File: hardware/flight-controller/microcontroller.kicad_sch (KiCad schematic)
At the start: 49 parts, among them J10 Conn_01x05, J8 IDC-6, J9 IDC-10, SW2 SW_Push, U4 STM32U535RET6, U5 ESP-12E, Y1 8 MHz

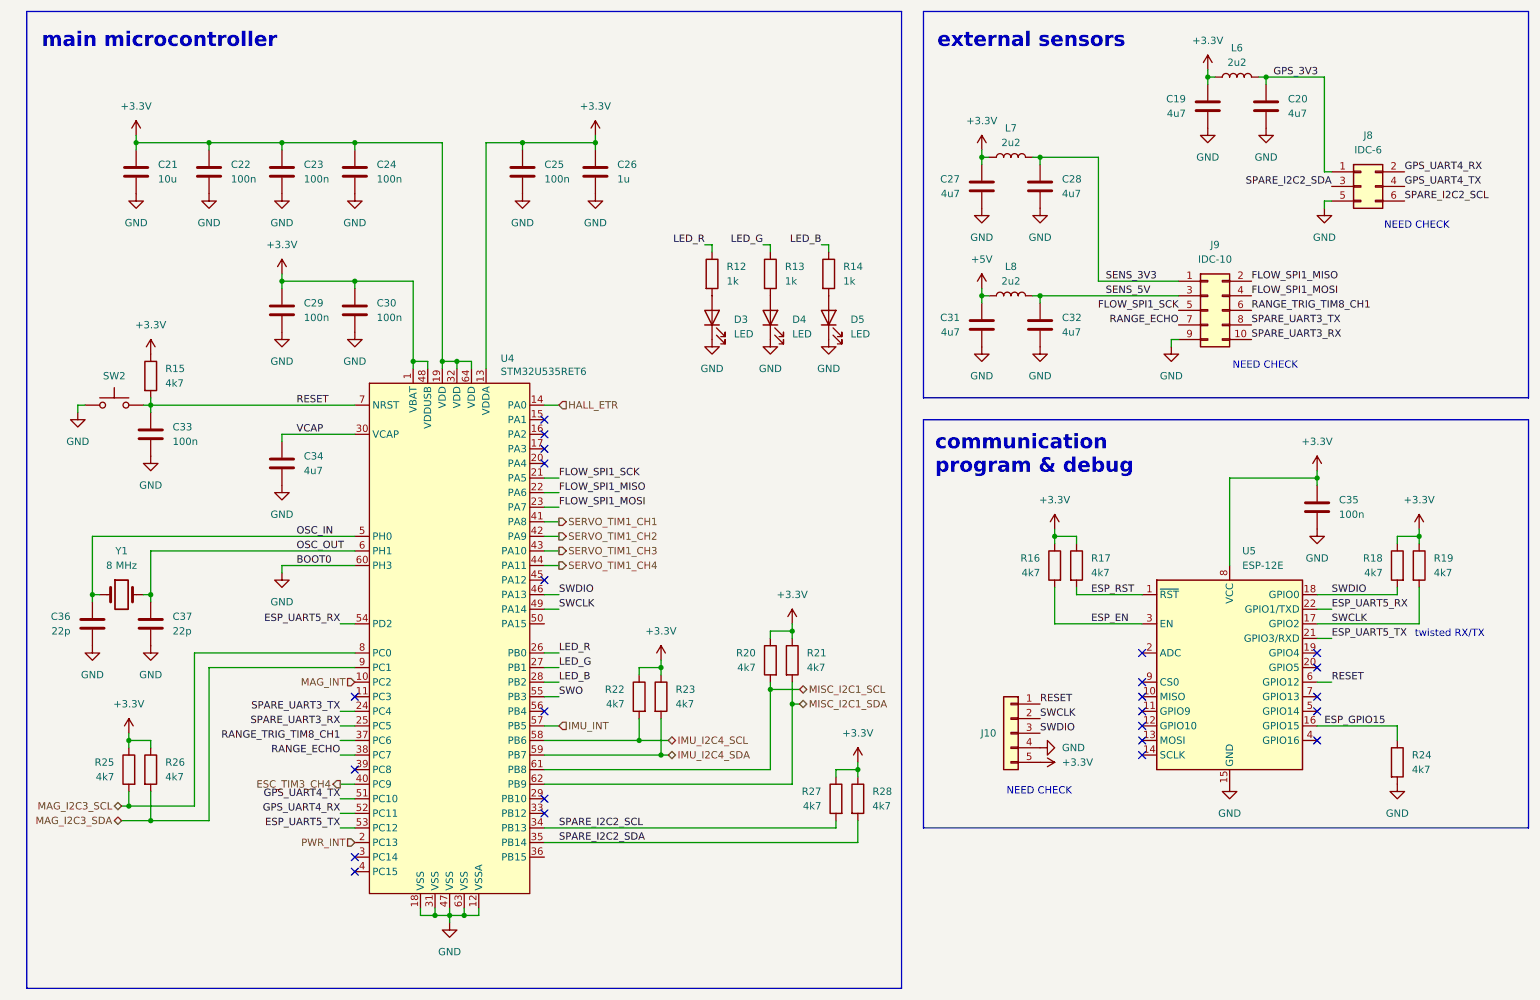
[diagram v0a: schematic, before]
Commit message: schematic cleanup
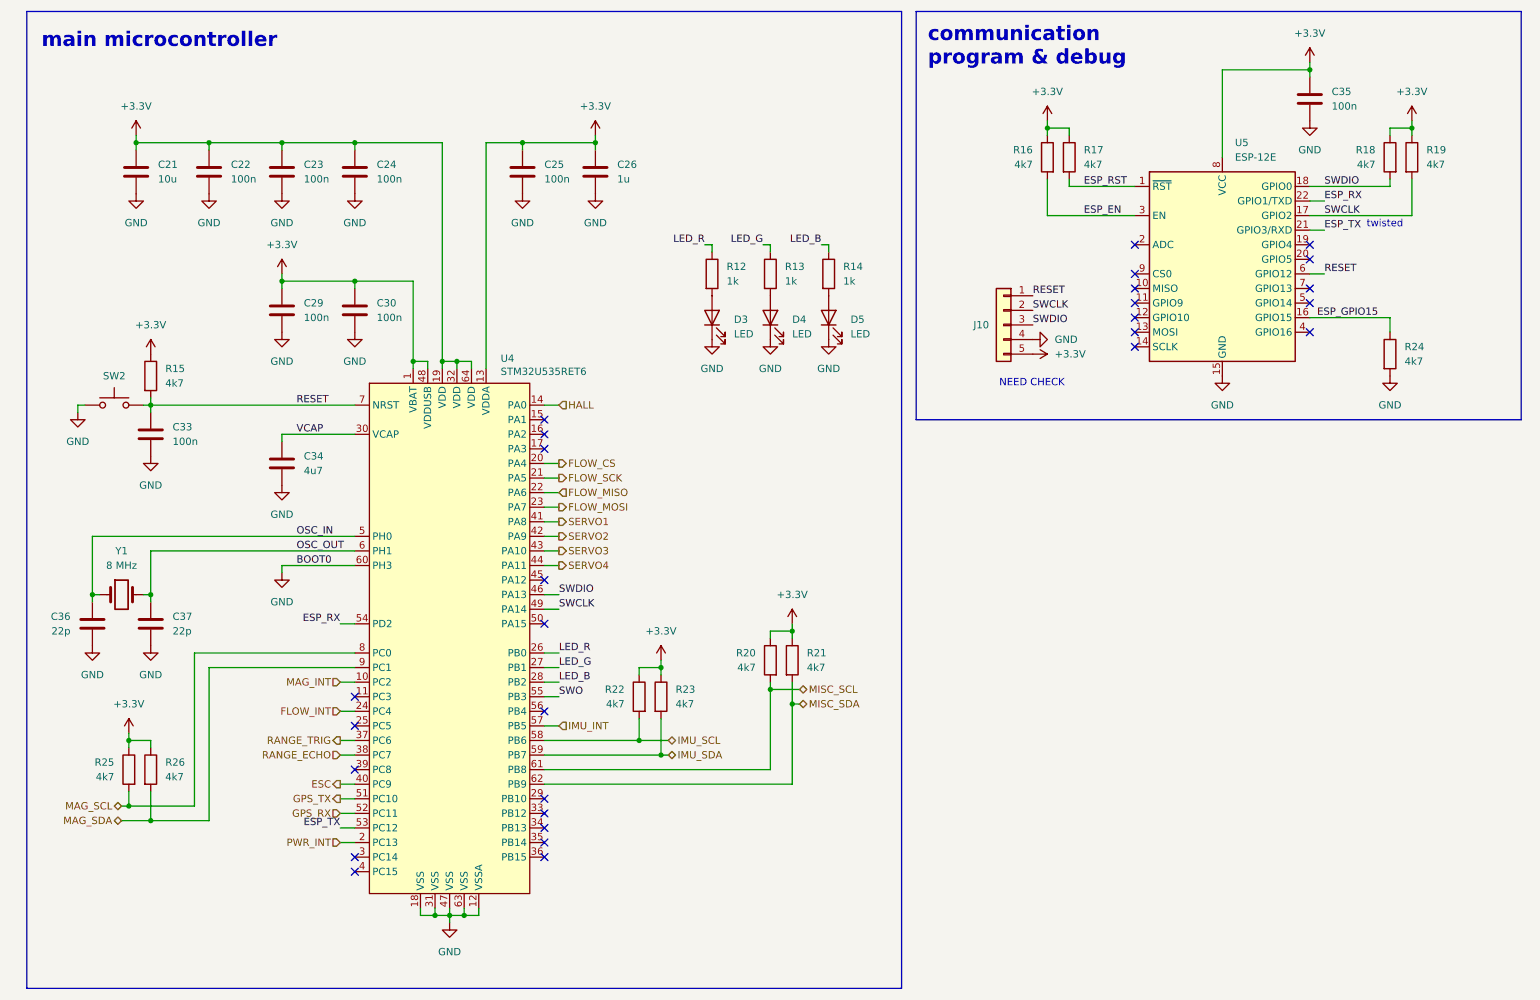
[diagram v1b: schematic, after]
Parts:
- removed C19, C20, C27, C28, C31, C32: 4u7, symbol Device:C
- removed J8: IDC-6, symbol Connector_Generic:Conn_02x03_Odd_Even
- removed J9: IDC-10, symbol Connector_Generic:Conn_02x05_Odd_Even
- removed L6, L7, L8: 2u2, symbol Device:L
- removed R27, R28: 4k7, symbol Device:R
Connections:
- net FLOW_CS: now reaches U4.20 (PA4)
- net ESC_TIM3_CH4 renamed ESC
- net ESP_UART5_RX renamed ESP_RX
- net ESP_UART5_TX renamed ESP_TX
- net FLOW_SPI1_MISO renamed FLOW_MISO
- net FLOW_SPI1_MOSI renamed FLOW_MOSI
- net FLOW_SPI1_SCK renamed FLOW_SCK
- net GPS_UART4_RX renamed GPS_RX
- net GPS_UART4_TX renamed GPS_TX
- net HALL_ETR renamed HALL
- net IMU_I2C4_SCL renamed IMU_SCL
- net IMU_I2C4_SDA renamed IMU_SDA
- net MAG_I2C3_SCL renamed MAG_SCL
- net MAG_I2C3_SDA renamed MAG_SDA
- net MISC_I2C1_SCL renamed MISC_SCL
- net MISC_I2C1_SDA renamed MISC_SDA
- net RANGE_TRIG_TIM8_CH1 renamed RANGE_TRIG
- net SERVO_TIM1_CH1 renamed SERVO1
- net SERVO_TIM1_CH2 renamed SERVO2
- net SERVO_TIM1_CH3 renamed SERVO3
- net SERVO_TIM1_CH4 renamed SERVO4
- net SPARE_I2C2_SCL: no longer names the net of U4.34 (PB13)
- net SPARE_I2C2_SDA: no longer names the net of U4.35 (PB14)
- net SPARE_UART3_RX: no longer names the net of U4.25 (PC5)
- net SPARE_UART3_TX renamed FLOW_INT
- no-connect marks 24 -> 28
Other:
- note added: "twisted"
- note removed: "external sensors"
- note removed: "twisted RX/TX"
- moved on the sheet: C35, J10, R16, R17, R18, R19, R24, U5

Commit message: still working
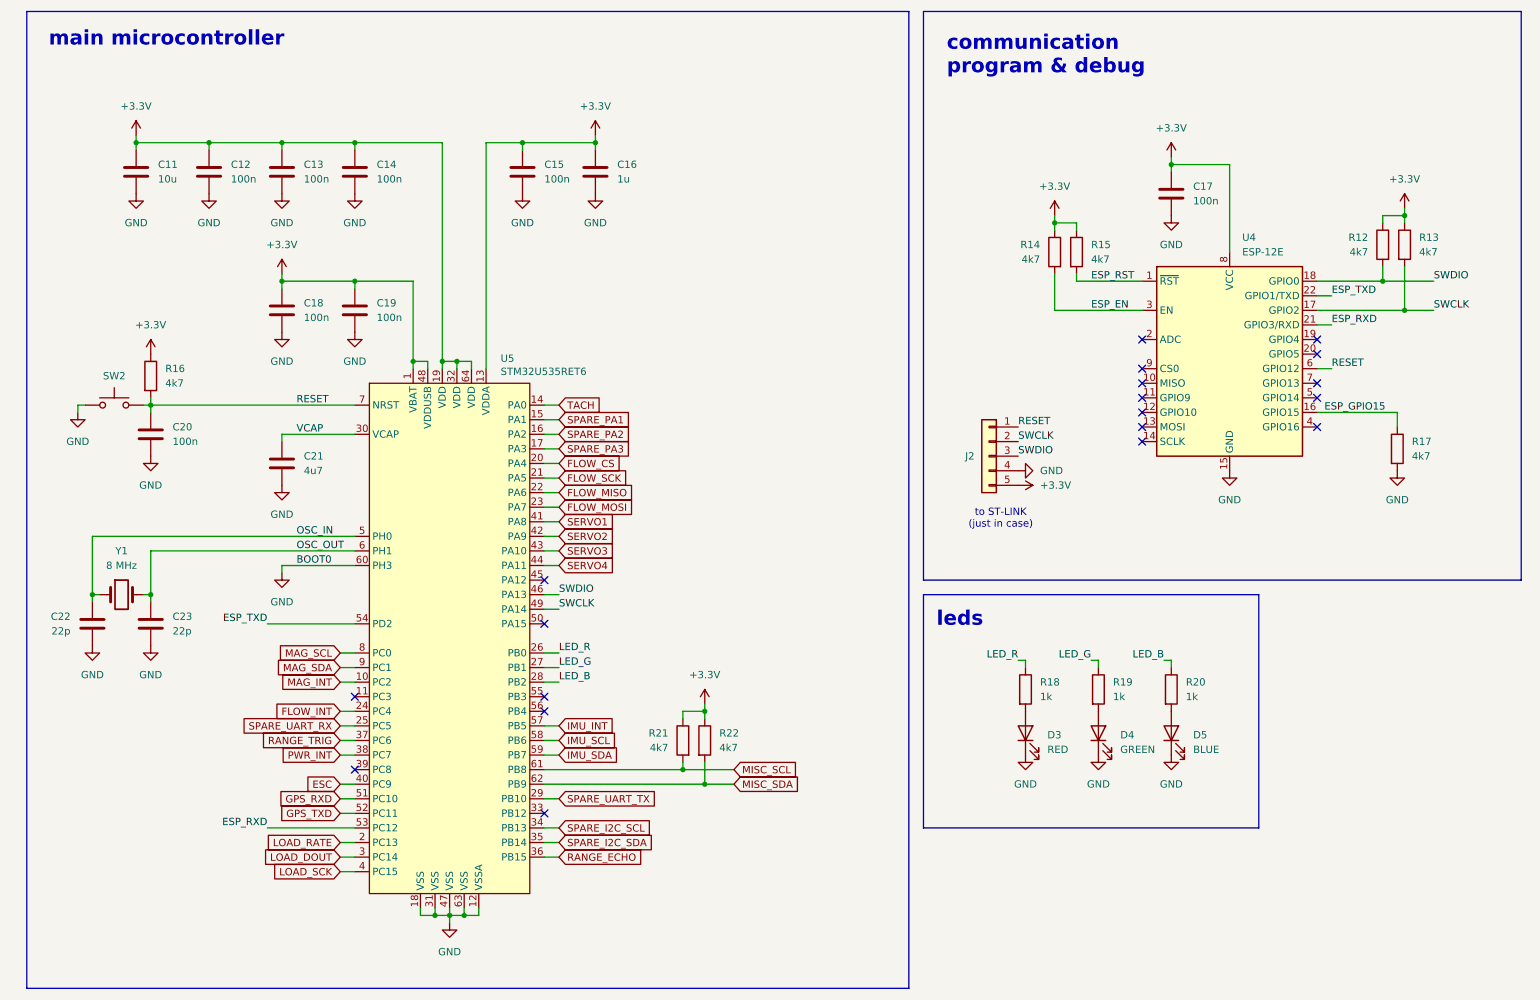
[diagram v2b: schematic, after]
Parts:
- removed R12, R13, R14: 1k, symbol Device:R
- removed R22, R23, R25, R26: 4k7, symbol Device:R
- added R18, R19, R20: 1k, Resistor_SMD:R_0603_1608Metric, symbol Device:R
- C12: renamed from C22; footprint (none) -> Capacitor_SMD:C_0603_1608Metric
- C13: renamed from C23; footprint (none) -> Capacitor_SMD:C_0603_1608Metric
- C14: renamed from C24; footprint (none) -> Capacitor_SMD:C_0603_1608Metric
- C15: renamed from C25; footprint (none) -> Capacitor_SMD:C_0603_1608Metric
- C17: renamed from C35; footprint (none) -> Capacitor_SMD:C_0603_1608Metric
- C18: renamed from C29; footprint (none) -> Capacitor_SMD:C_0603_1608Metric
- C19: renamed from C30; footprint (none) -> Capacitor_SMD:C_0603_1608Metric
- C20: renamed from C33; footprint (none) -> Capacitor_SMD:C_0603_1608Metric
- C22: renamed from C36; footprint (none) -> Capacitor_SMD:C_0603_1608Metric
- C23: renamed from C37; footprint (none) -> Capacitor_SMD:C_0603_1608Metric
- D3: value LED -> RED; footprint (none) -> LED_SMD:LED_0603_1608Metric
- D4: value LED -> GREEN; footprint (none) -> LED_SMD:LED_0603_1608Metric
- D5: value LED -> BLUE; footprint (none) -> LED_SMD:LED_0603_1608Metric
- J2: renamed from J10; footprint (none) -> Connector_PinHeader_2.54mm:PinHeader_1x05_P2.54mm_Vertical
- R12: renamed from R18; footprint (none) -> Resistor_SMD:R_0603_1608Metric
- R13: renamed from R19; footprint (none) -> Resistor_SMD:R_0603_1608Metric
- R14: renamed from R16; footprint (none) -> Resistor_SMD:R_0603_1608Metric
- R15: renamed from R17; footprint (none) -> Resistor_SMD:R_0603_1608Metric
- R16: renamed from R15; footprint (none) -> Resistor_SMD:R_0603_1608Metric
- R17: renamed from R24; footprint (none) -> Resistor_SMD:R_0603_1608Metric
- R21: renamed from R20; footprint (none) -> Resistor_SMD:R_0603_1608Metric
- R22: renamed from R21; footprint (none) -> Resistor_SMD:R_0603_1608Metric
- Y1: footprint (none) -> Crystal:Crystal_SMD_5032-2Pin_5.0x3.2mm
- renumbered C21 to C11, C26 to C16, C34 to C21, U5 to U4, U4 to U5
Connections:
- net LED_B: now also R20.1
- net LED_G: now also R19.1
- net LED_R: now also R18.1
- net PWR_INT: now also U5.38 (PC7); no longer U5.2 (PC13)
- net RANGE_ECHO: now also U5.36 (PB15); no longer U5.38 (PC7)
- net at D3.2 (A): now also R18.2
- net at D5.2 (A): now also R20.2
- net at D4.2 (A): now also R19.2
- net SPARE_PA1: now reaches U5.15 (PA1)
- net SPARE_PA2: now reaches U5.16 (PA2)
- net SPARE_PA3: now reaches U5.17 (PA3)
- net SPARE_UART_RX: now reaches U5.25 (PC5)
- net SPARE_UART_TX: now reaches U5.29 (PB10)
- net LOAD_DOUT: now reaches U5.3 (PC14)
- net SPARE_I2C_SCL: now reaches U5.34 (PB13)
- net SPARE_I2C_SDA: now reaches U5.35 (PB14)
- net LOAD_SCK: now reaches U5.4 (PC15)
- net ESP_RX renamed ESP_TXD
- net ESP_TX renamed ESP_RXD
- net GPS_RX renamed GPS_TXD
- net GPS_TX renamed GPS_RXD
- net HALL renamed TACH
- net SWO: no longer names the net of U5.55 (PB3)
- new net LOAD_RATE: U5.2 (PC13)
- no-connect marks 28 -> 19
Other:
- note added: "leds"
- note added: "to ST-LINK (just in case)"
- note removed: "NEED CHECK"
- note removed: "twisted"
- moved on the sheet: C17, J2, R12, R13, R14, R15, R17, R21, R22, U4
